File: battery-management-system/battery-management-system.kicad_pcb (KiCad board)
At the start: 4 copper layers, 130 x 100 mm, 216 parts, among them J1 CELL4_PLUS, J10 9V4, J11 5V, J12 18V, J13 3V3, J14 AMPHENOL_micro_usb_10118194-0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, J16 I2C, J17 UART_INTERCONNECT, J18 LEDS, J19 CHARGE/DISCHARGE, J2 CELL4_MINUS, J20 UART_USB, J21 rspro_header_5pin_3_5mm, J22 TEMP_CELL1, J23 TEMP_CELL2, J24 TEMP_CELL3, J25 TEMP_CELL4, J26 BALANCE_CONTROL, J27 BALANCE_INPUTS, J28 BALANCE_CURRENT, J3 CELL3_MINUS, J4 CELL2_MINUS, J5 CELL1_MINUS, J6 VBAT+, J7 VBAT+_CHARGE, J8 VBAT-, J9 -5V, Q1 DMN3730U, Q10 BS250FTA, Q11 BS250FTA, Q12 BS250FTA, Q13 BS250FTA, Q14 DMN3730U, Q15 DMN3404L, Q16 DMN3730U, Q17 DMN3730U, Q18 DMN3730U, Q19 DMN3730U, Q2 TJ40S04M3L, Q3 TJ40S04M3L, Q4 DMN3730U, Q5 DMN3730U, Q6 DMN3730U, Q7 DMN3730U, Q8 DMN3730U, Q9 DMN3730U, SW1 CELL4_PLUS, SW2 CELL4_MINUS, SW3 CELL3_PLUS, SW4 CELL3_MINUS, SW5 CELL2_PLUS, SW6 CELL2_MINUS, SW7 CELL1_PLUS, SW8 CELL1_MINUS, U1 ICL7660, U10 STC3100, U11 STM32L071CZTx, U12 LM2904M8-13, U13 LM2904M8-13, U14 LM2904M8-13, U15 LM2904M8-13, U16 MC74VHC139, U2 ICL7660, U3 L6982C33DR, U4 L6982C33DR, U5 ICL7660, U6 FT230XS, U7 ARM-JTAG-SWD, U8 AT24C512C, U9 NCT75DR2G

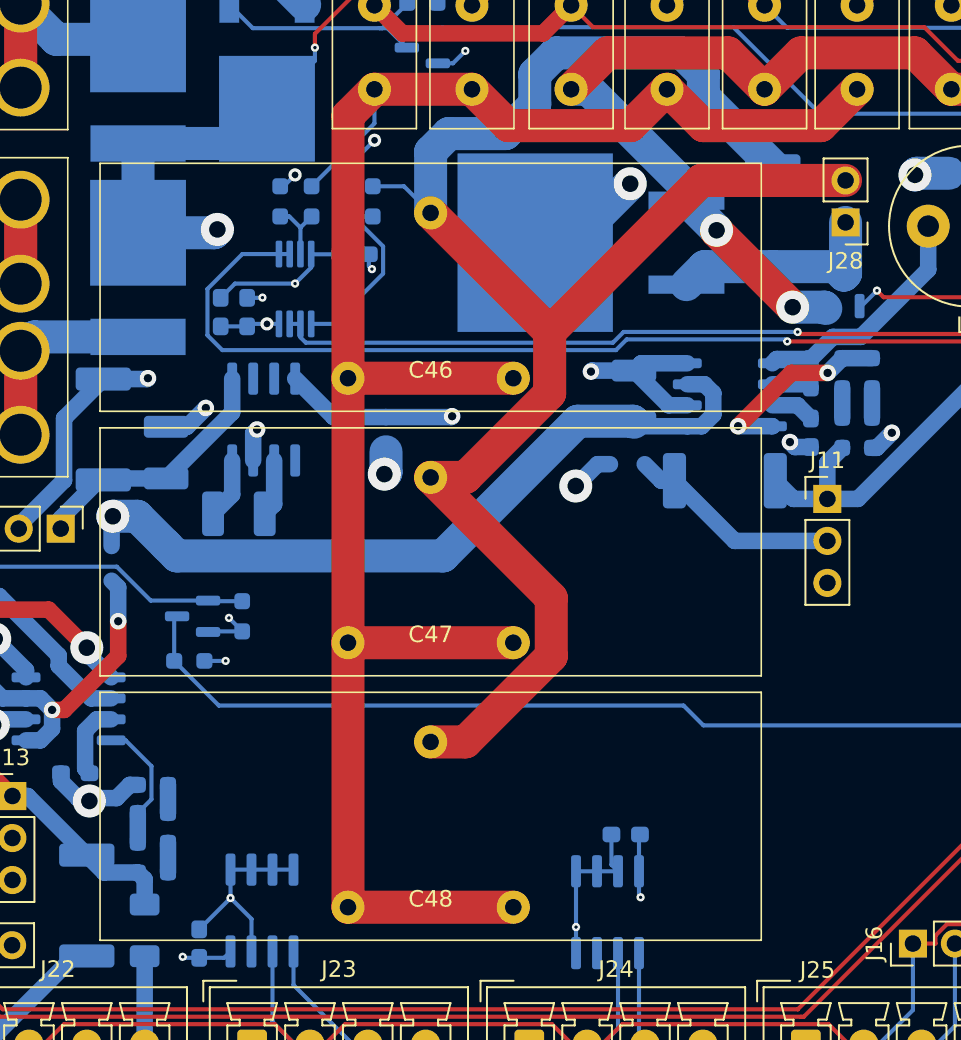
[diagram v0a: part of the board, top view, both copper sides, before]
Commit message: update footprints and layout
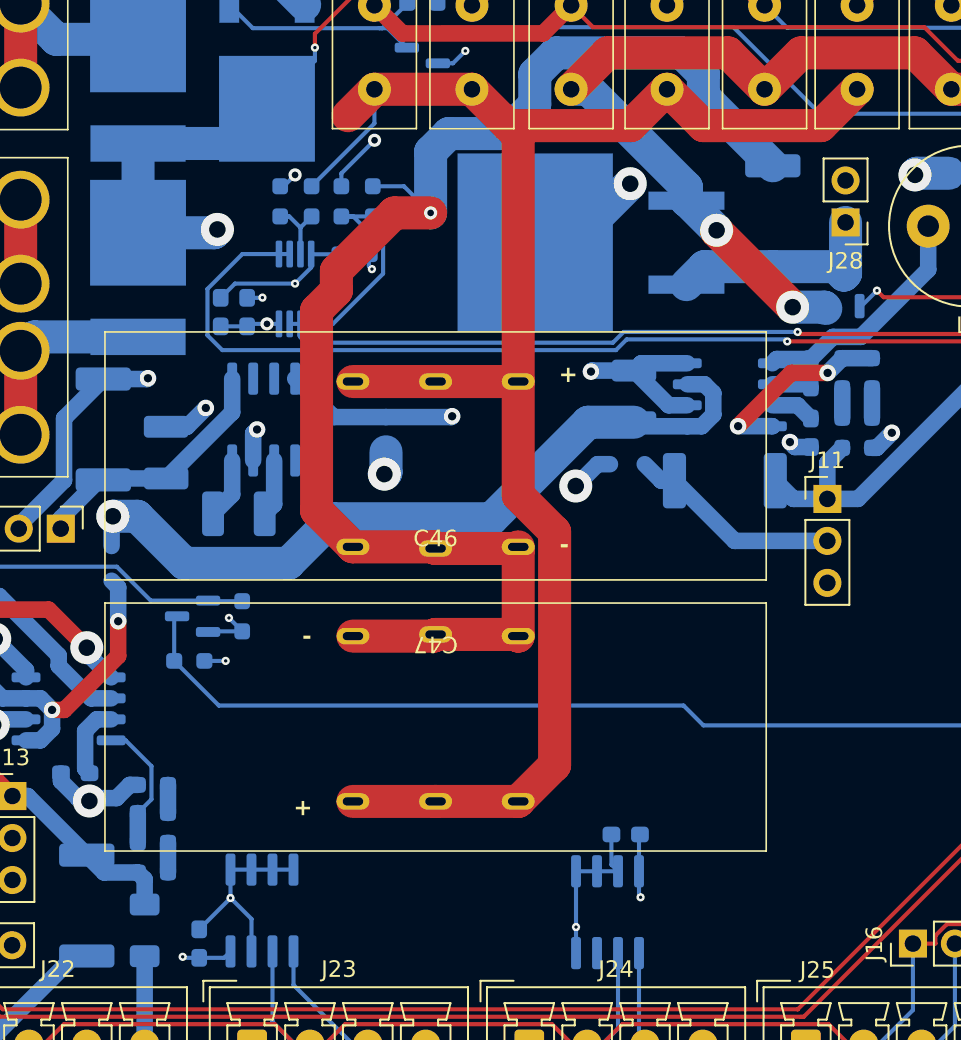
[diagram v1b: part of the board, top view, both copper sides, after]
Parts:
- removed C48: 90F, benediktibk:vishay_super_cap_form_g
- moved C46 10.2 mm to (67.1, 84.0)
- moved C47 0.50 mm to (67.1, 89.4), turned to 180 degrees
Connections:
- C46 pad 1: /BALANCE_CAP_MINUS_RAW -> /BALANCE_CAP_PLUS_RAW
- C46 pad 2: /BALANCE_CAP_PLUS_RAW -> /BALANCE_CAP_MINUS_RAW
- C47 pad 1: /BALANCE_CAP_MINUS_RAW -> /BALANCE_CAP_PLUS_RAW
- C47 pad 2: /BALANCE_CAP_PLUS_RAW -> /BALANCE_CAP_MINUS_RAW
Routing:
- net /BALANCE_CAP_MINUS_RAW: track 103.9 -> 86.5 mm, vias 0 -> 1
- net /BALANCE_CAP_PLUS_RAW: track 120.4 -> 105.5 mm
